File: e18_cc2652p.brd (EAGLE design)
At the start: 23.4 x 14.8 mm, 44 parts, among them IC3 CC2652R1FRGZ, Q1 32.768kHz, U1 MX25R8035FZUIL0, Y1 Q22FA12800150

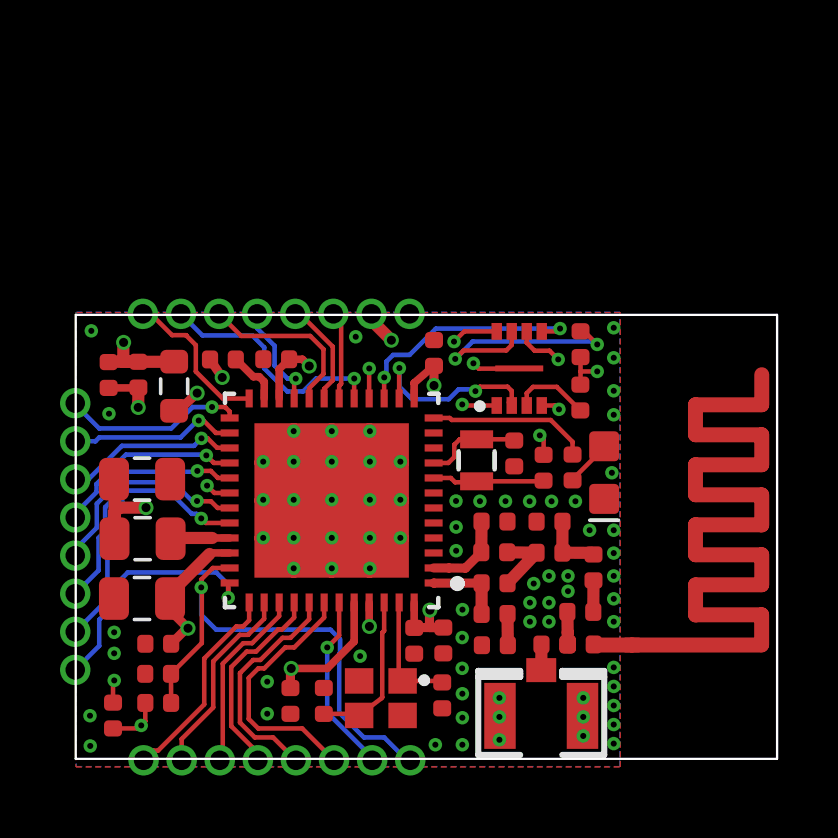
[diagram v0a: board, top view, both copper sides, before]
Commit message: Add files via upload
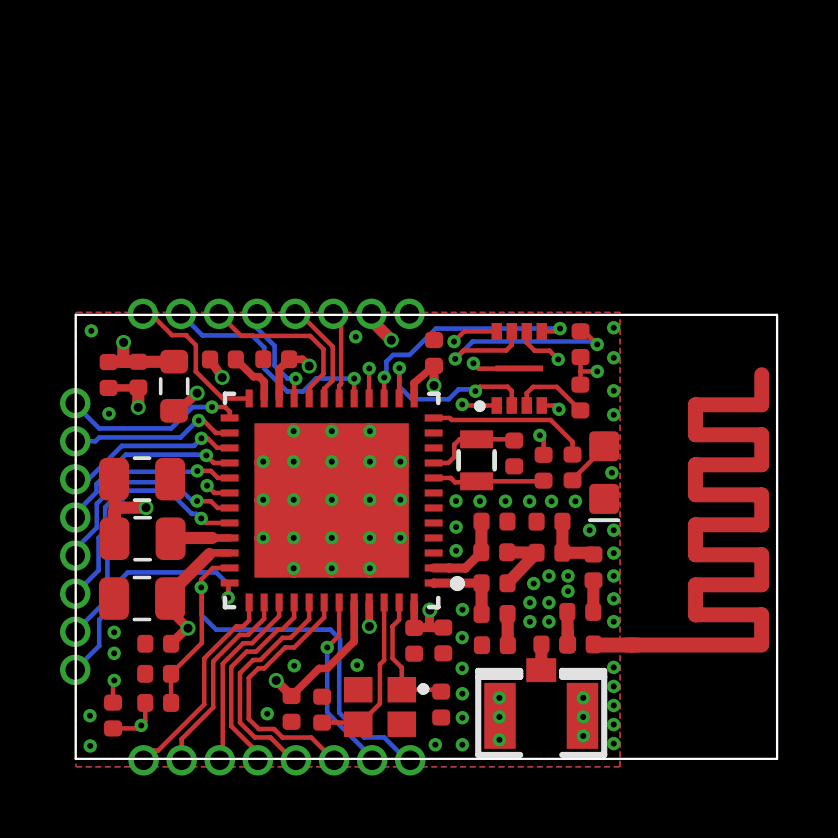
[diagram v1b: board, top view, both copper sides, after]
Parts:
- moved C22 0.31 mm to (12.2, 1.80)
- moved C20 0.30 mm to (8.23, 1.63)
- moved Y1 0.29 mm to (10.2, 1.72)
- moved C13 0.27 mm to (7.21, 1.65)
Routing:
- net N$15: track 4.02 -> 4.70 mm

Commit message: Add files via upload
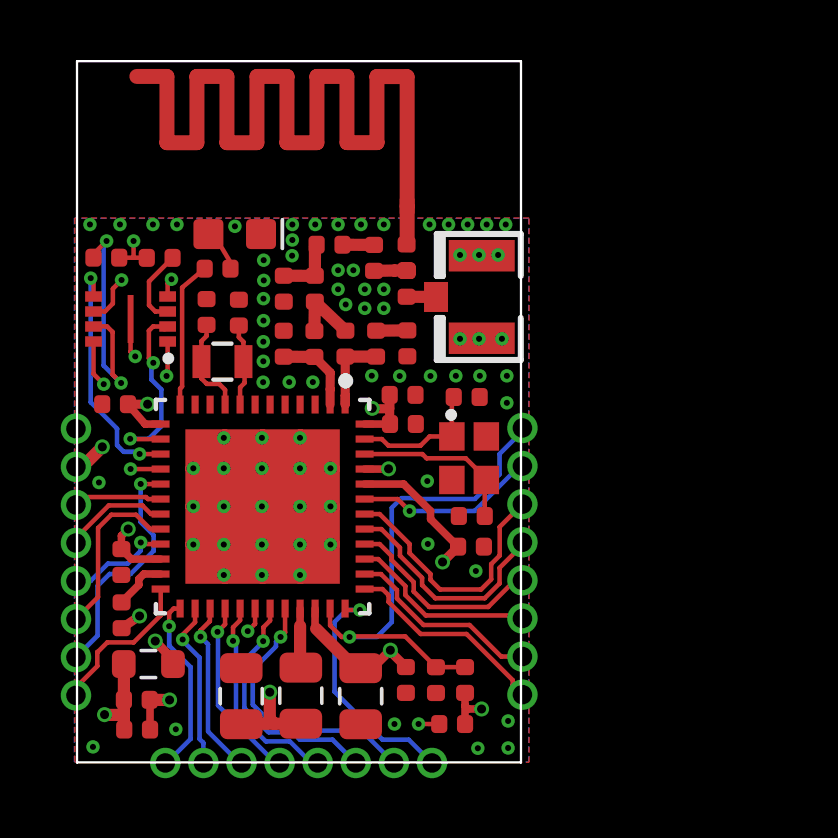
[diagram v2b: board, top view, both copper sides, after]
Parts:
- moved U$1 16.1 mm to (11.0, 18.2), turned to 0 degrees
- moved R2 16.1 mm to (1.04, 16.7), turned to 0 degrees
- moved R4 14.8 mm to (2.81, 16.7), turned to 0 degrees
- moved G 14.7 mm to (5.32, 17.5), turned to 0 degrees
- moved C21 14.1 mm to (11.0, 16.7), turned to 89.6 degrees
- moved X1 14.1 mm to (13.6, 15.4), turned to 180 degrees
- moved L6 13.9 mm to (8.48, 17.1), turned to 0 degrees
- moved C19 13.7 mm to (9.96, 16.7), turned to 270 degrees
- moved R5 13.6 mm to (4.75, 16.3), turned to 0 degrees
- moved U1 13.1 mm to (1.84, 14.6), turned to 180 degrees
- moved C23 13.0 mm to (11.0, 15.8), turned to 270 degrees
- moved J3 12.9 mm to (0.02, 2.10), turned to 90 degrees
- moved J1 12.8 mm to (14.9, 2.13), turned to 90 degrees
- moved J2 12.4 mm to (3.00, -0.15), turned to 0 degrees
- moved C2 11.9 mm to (2.06, 0.96), turned to 180 degrees
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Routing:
- net GND: track 6.84 -> 5.86 mm, vias 81 -> 82
- net X32K_Q1: track 3.75 -> 2.78 mm
- net VDDR: track 7.92 -> 7.04 mm
- net CS: track 21.3 -> 20.5 mm
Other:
- board size 23.4 x 14.8 mm -> 14.8 x 23.4 mm
- board text added: "DIO16"
- board text added: "DIO17"
- board text added: "RESET"
- board text added: "RX/DIO12"
- board text added: "SBL/DIO15"
- board text added: "TX/DIO13"
- board text removed: "DIO12"
- board text removed: "DIO13"
- board text removed: "DIO15"
- board text removed: "RST"
- board text removed: "TDI"
- board text removed: "TDO"
